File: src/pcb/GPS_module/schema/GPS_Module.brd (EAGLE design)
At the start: 23.8 x 27.9 mm, 10 parts, among them J2 U.FL-R-SMT(01), U1 SL876Q5A001T001000

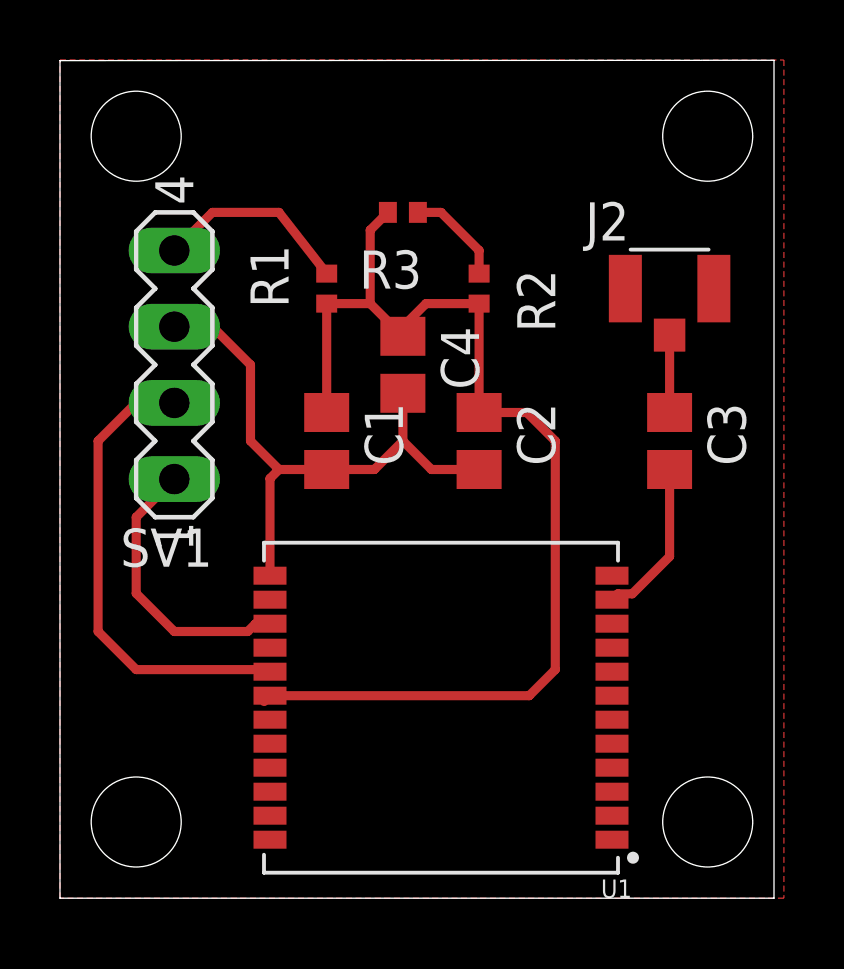
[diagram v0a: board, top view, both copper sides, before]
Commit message: Updated text for pcb
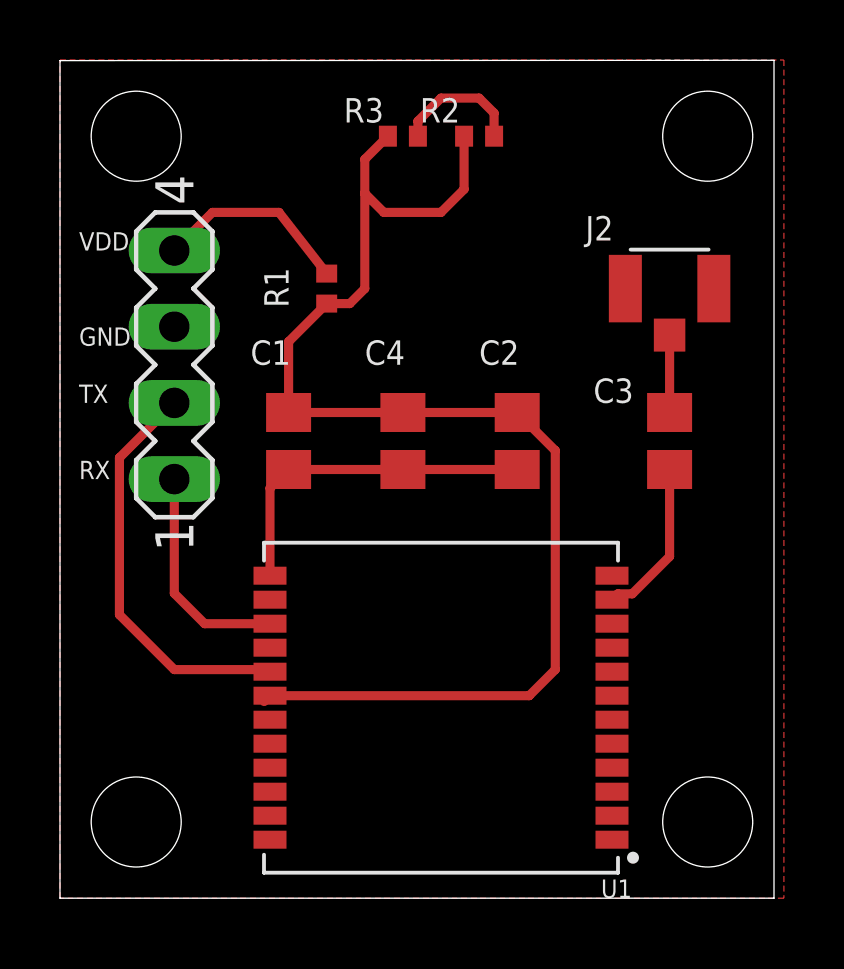
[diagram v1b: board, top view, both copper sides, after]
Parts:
- moved R2 5.08 mm to (14.0, 36.8), turned to 180 degrees
- moved C4 2.54 mm to (11.4, 26.7)
- moved R3 2.54 mm to (11.4, 36.8)
- moved C1 1.27 mm to (7.62, 26.7)
- moved C2 1.27 mm to (15.2, 26.7)
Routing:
- net GND: track 23.0 -> 15.8 mm
- net VIN: track 37.3 -> 43.9 mm
- net TX: track 15.7 -> 13.6 mm
- net RX: track 9.43 -> 7.42 mm
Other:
- board text added: "GND"
- board text added: "RX"
- board text added: "TX"
- board text added: "VDD"
